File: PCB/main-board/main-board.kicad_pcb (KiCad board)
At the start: 2 copper layers, 39 parts, among them J1 Conn_01x02_Pin, Q1 PN2222A, SW1 RotaryEncoder_Switch_MP, U1 LM358, U2 IRLIZ44N, U3 L7805

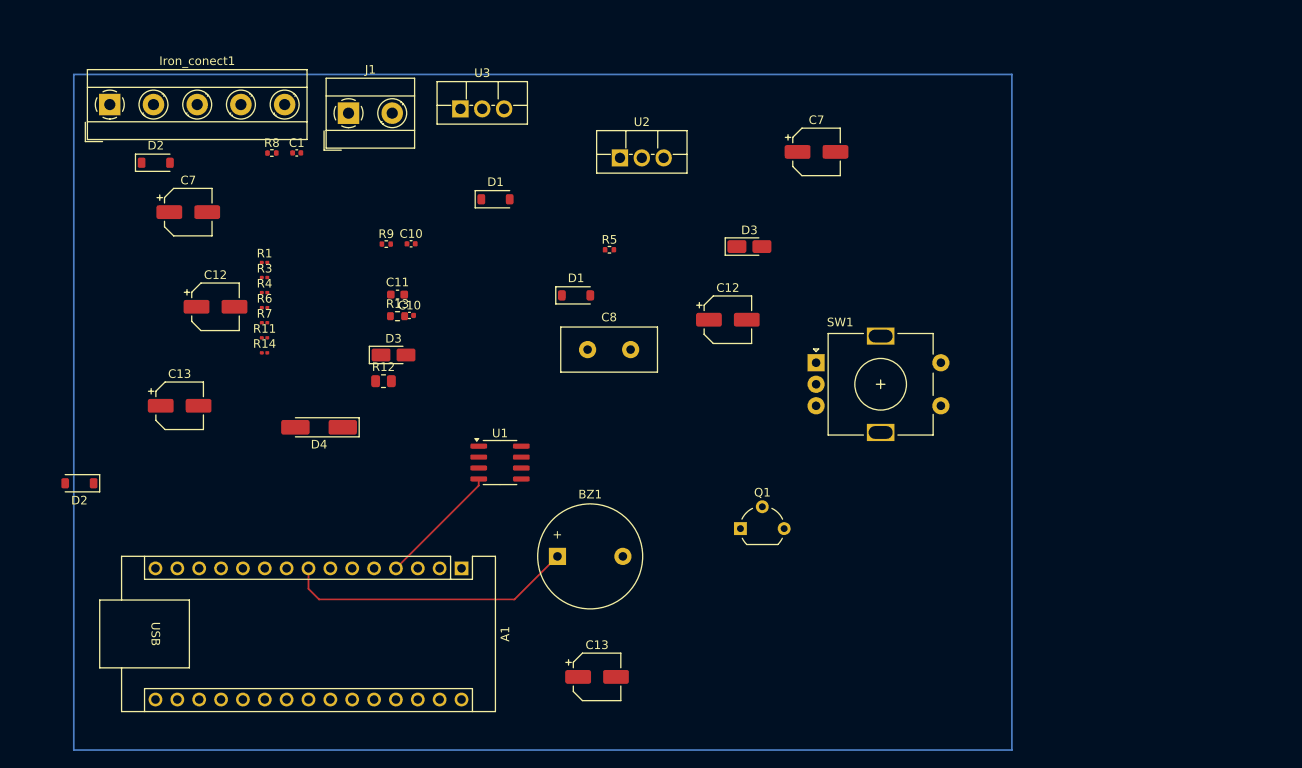
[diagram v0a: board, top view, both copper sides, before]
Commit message: update
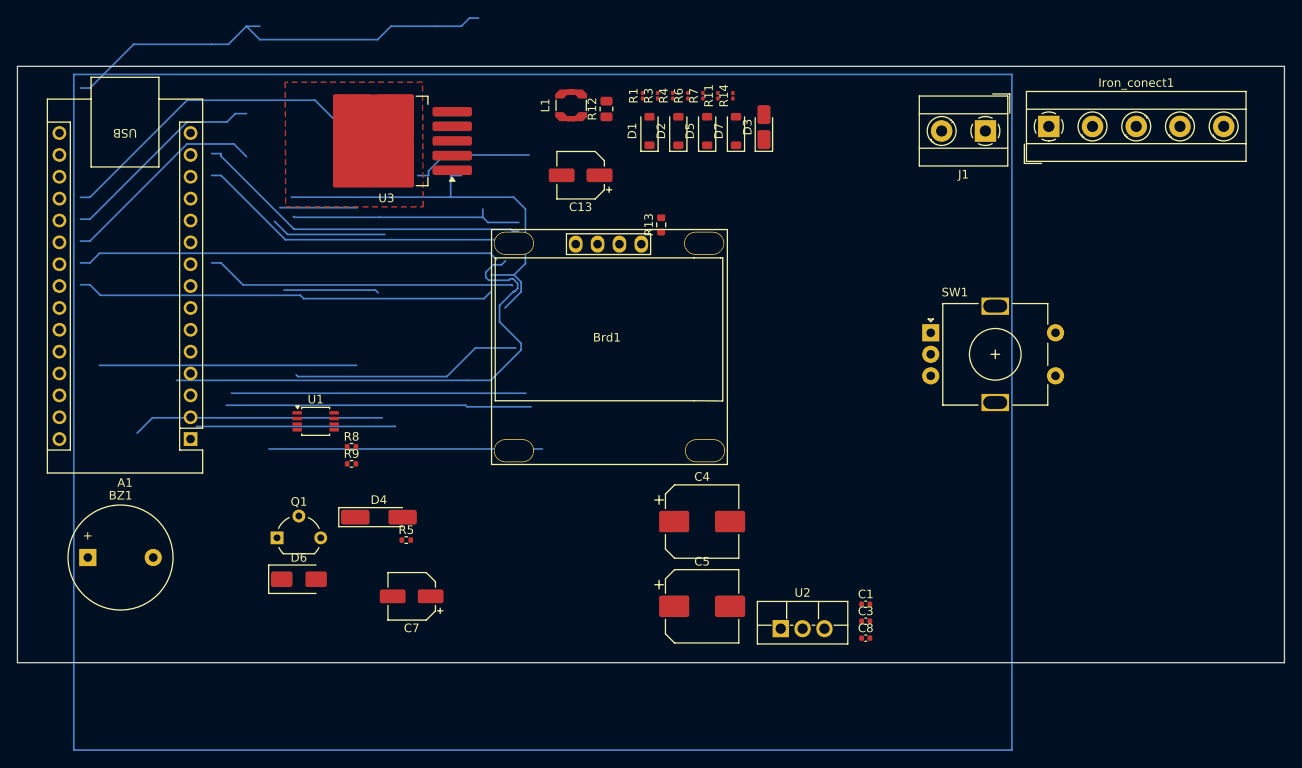
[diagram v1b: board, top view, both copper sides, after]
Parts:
- removed C10 (x2): 100nF, Capacitor_SMD:C_0402_1005Metric
- removed C11: 330nF, Capacitor_SMD:C_0603_1608Metric
- removed C12 (x2): 10uf 35v, Capacitor_SMD:CP_Elec_5x4.4
- removed the C13 at (139.8, 119.0)
- removed the C13 at (91.3, 87.5)
- removed the C7 at (165.3, 58.0)
- removed the C7 at (92.3, 65.0)
- removed the D1 at (137.4, 74.7)
- removed the D1 at (128.0, 63.5)
- removed the D2 at (79.7, 96.5)
- removed the D2 at (88.5, 59.3)
- removed the D3 at (157.5, 69.0)
- removed the D3 at (116.2, 81.6)
- added Brd1: SSD1306, library:128x64OLED, F.Cu at (140.9, 79.3)
- added C13: 10µF, Capacitor_SMD:CP_Elec_5x4.4, F.Cu at (137.9, 60.7)
- added C3: 100nf, Capacitor_SMD:C_0402_1005Metric, F.Cu at (171.0, 112.5)
- added C4: 220uf, Capacitor_SMD:CP_Elec_8x10, F.Cu at (152.0, 101.0)
- added C5: 220uf, Capacitor_SMD:CP_Elec_8x10, F.Cu at (152.0, 110.8)
- added C7: 10uf 35V, Capacitor_SMD:CP_Elec_5x4.4, F.Cu at (118.3, 109.6)
- added D1: 1N5819, Diode_SMD:D_SOD-123, F.Cu at (145.9, 55.6)
- added D2: 1N4007, Diode_SMD:D_SOD-123, F.Cu at (149.2, 55.6)
- added D3: 5V, Diode_SMD:D_MicroMELF_Handsoldering, F.Cu at (159.2, 55.1)
- added D5: 1N4007, Diode_SMD:D_SOD-123, F.Cu at (152.6, 55.6)
- added D6: B120-E3, Diode_SMD:D_SMA, F.Cu at (105.2, 107.7)
- added D7: 1N4007, Diode_SMD:D_SOD-123, F.Cu at (155.9, 55.6)
- added L1: 330uH, Inductor_SMD:L_Coilcraft_LPS3314, F.Cu at (136.8, 52.6)
- C8: footprint Capacitor_THT:C_Disc_D11.0mm_W5.0mm_P5.00mm -> Capacitor_SMD:C_0402_1005Metric
- U1: footprint Package_SO:SOIC-8_3.9x4.9mm_P1.27mm -> Package_SO:TSSOP-8_3x3mm_P0.65mm
- U3: value L7805 -> LM2596S-5; footprint Package_TO_SOT_THT:TO-220F-3_Vertical -> Package_TO_SOT_SMD:TO-263-5_TabPin3
- moved Iron_conect1 109.1 mm to (192.3, 55.0)
- moved C1 84.4 mm to (171.0, 110.6)
- moved J1 74.0 mm to (184.9, 55.6), turned to 180 degrees
- moved R14 62.1 mm to (155.6, 51.5), turned to 90 degrees
- moved R11 59.7 mm to (153.8, 51.5), turned to 90 degrees
- moved U2 57.8 mm to (161.1, 113.4)
- moved R7 57.3 mm to (152.1, 51.5), turned to 90 degrees
- moved R6 55.0 mm to (150.3, 51.5), turned to 90 degrees
- moved BZ1 54.6 mm to (80.6, 105.1)
- moved Q1 53.9 mm to (102.6, 102.8)
- moved R4 52.7 mm to (148.6, 51.5), turned to 90 degrees
- moved R3 50.3 mm to (146.8, 51.5), turned to 90 degrees
- moved R1 48.0 mm to (145.1, 51.5), turned to 90 degrees
- moved C8 46.6 mm to (171.0, 114.5)
- moved R5 41.2 mm to (117.6, 103.1)
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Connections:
- C8 pad 1: unconnected-(C8-Pad1) -> Net-(D2-A)
- C8 pad 2: unconnected-(C8-Pad2) -> GND
- J1 pad 2: 24V+ -> +24V
- R12 pad 1: 24V+ -> +24V
- U2 pad 2: 24V+ -> +24V
- U3 pad 1: 24V+ -> Net-(D5-K)
- U3 pad 2: GND -> Net-(D6-K)
- U3 pad 3: VCC -> GND
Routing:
- net GND: track 14.4 -> 296.2 mm
- net D9: track 0.00 -> 86.5 mm
- net D10: track 0.00 -> 48.6 mm
- net unconnected-(A1-SCK-Pad16): track 0.00 -> 41.2 mm
- net A0: track 0.00 -> 36.1 mm
- net Net-(D2-A): track 0.00 -> 35.5 mm
- net Net-(U1A--): track 0.00 -> 34.2 mm
- net D5: track 33.9 -> 0.00 mm
- net unconnected-(A1-~{RESET}-Pad28): track 0.00 -> 29.9 mm
- net unconnected-(A1-RX1-Pad2): track 0.00 -> 29.2 mm
- net Net-(U1B-+): track 0.00 -> 27.0 mm
- net B: track 0.00 -> 24.6 mm
- net A: track 0.00 -> 24.4 mm
- net Net-(D7-A): track 0.00 -> 13.4 mm
- net VCC: track 0.00 -> 11.1 mm
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- added copper zone on F.Cu, net GND
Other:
- board outline added: 147.2 x 69.3 mm
